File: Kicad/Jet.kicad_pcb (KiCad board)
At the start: 2 copper layers, 17 parts, among them J1 Conn_02x13_Odd_Even, J2 Conn_01x03_Female, J3 POWER, J4 Conn_02x10_Odd_Even, J5 Conn_02x10_Odd_Even, Q1 Q_NPN_EBC, Q2 Q_NPN_EBC, U1 PC817, U2 PC817

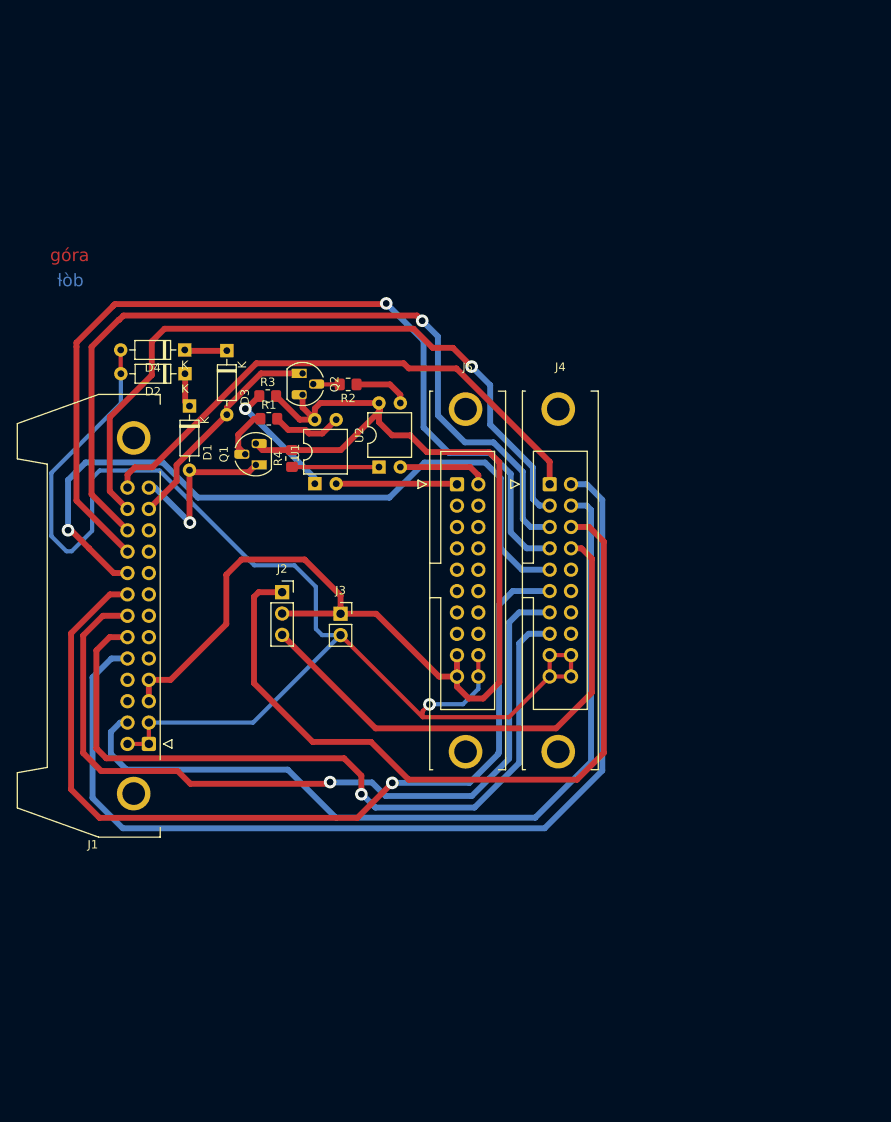
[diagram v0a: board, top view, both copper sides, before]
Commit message: UPDATE: footprint
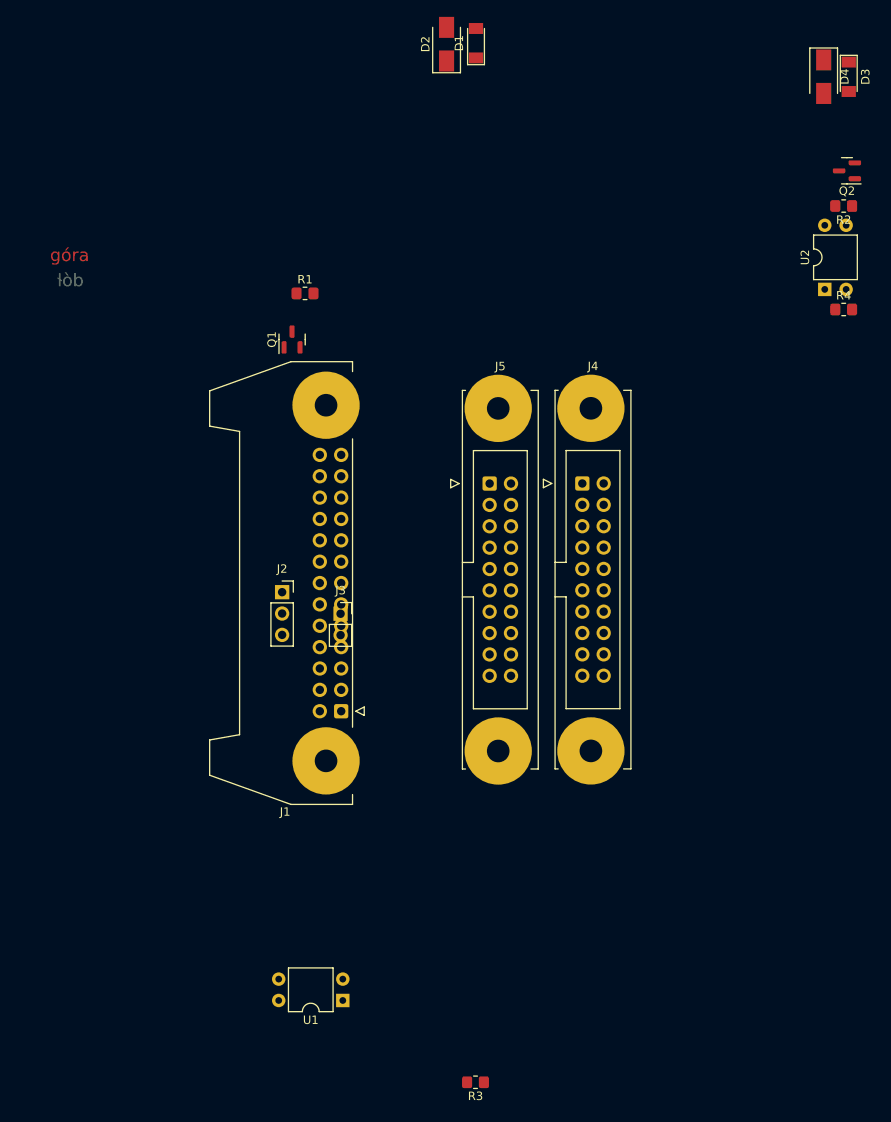
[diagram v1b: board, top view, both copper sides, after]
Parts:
- D1, D3: value D_Zener -> BZM55C30-LGE; footprint Diode_THT:D_DO-35_SOD27_P7.62mm_Horizontal -> Diode_SMD:D_MiniMELF
- D2, D4: value 1N4448 -> M7L-DIO; footprint Diode_THT:D_DO-35_SOD27_P7.62mm_Horizontal -> Diode_SMD:D_SMA
- Q1, Q2: value Q_NPN_EBC -> BCW66FR; footprint Package_TO_SOT_THT:TO-92L_HandSolder -> Package_TO_SOT_SMD:SOT-23
- moved R3 85.3 mm to (112.6, 149.2), turned to 180 degrees
- moved D4 82.6 mm to (154.0, 29.6), turned to -90 degrees
- moved D3 80.8 mm to (156.9, 29.6)
- moved Q2 69.1 mm to (156.7, 40.8), turned to 180 degrees
- moved R4 68.0 mm to (156.3, 57.3), turned to 0 degrees
- moved R2 62.6 mm to (156.3, 45.0)
- moved U1 61.5 mm to (96.8, 139.5), turned to 180 degrees
- moved U2 57.1 mm to (154.1, 54.9)
- moved D1 55.0 mm to (112.6, 25.6), turned to 90 degrees
- moved D2 50.0 mm to (109.1, 25.8), turned to 90 degrees
- moved J1 23.2 mm to (96.6, 105.1)
- moved Q1 15.5 mm to (90.8, 60.9)
- moved R1 15.5 mm to (92.3, 55.4)
- moved J4 3.88 mm to (125.3, 78.0)
- moved J5 3.88 mm to (114.2, 78.0)
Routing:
- net GND: track 165.1 -> 0.00 mm, vias 1 -> 0
- net VCC: track 154.0 -> 0.00 mm
- net IN_AGREGAT_REKA: track 121.1 -> 0.00 mm
- net IN_AGREGAT_KRANCOWKA: track 107.8 -> 0.00 mm, vias 1 -> 0
- net IN_CONFIG2: track 107.0 -> 0.00 mm, vias 1 -> 0
- net IN_AGREGAT_RESET: track 100.6 -> 0.00 mm
- net IN_KOLO_KRANCOWKA: track 98.8 -> 0.00 mm, vias 1 -> 0
- net IN_INTERWAL: track 96.5 -> 0.00 mm, vias 1 -> 0
- net TIME+: track 91.3 -> 0.00 mm
- net IN_WANNA: track 91.0 -> 0.00 mm, vias 1 -> 0
- net IN_CONFIG1: track 86.9 -> 0.00 mm, vias 1 -> 0
- net IN_START: track 84.5 -> 0.00 mm, vias 1 -> 0
- net IN_OBUDOWA: track 64.7 -> 0.00 mm
- net TIME-: track 62.3 -> 0.00 mm
- net AGREGAT: track 26.6 -> 0.00 mm
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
